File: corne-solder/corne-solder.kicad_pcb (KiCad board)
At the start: 2 copper layers, 133.8 x 91.9 mm, 47 parts, among them J1 Battery Connector, J2 nice!view, SW1 SW_Push, SW10 SW_Push, SW11 SW_Push, SW12 SW_Push, SW13 SW_Push, SW14 SW_Push, SW15 SW_Push, SW16 SW_Push, SW17 SW_Push, SW18 SW_Push, SW19 SW_Push, SW2 SW_Push, SW20 SW_Push, SW21 SW_Push, SW3 SW_Push, SW4 SW_Push, SW5 SW_Push, SW6 SW_Push, SW7 SW_Push, SW8 SW_Push, SW9 SW_Push, U1 ProMicro

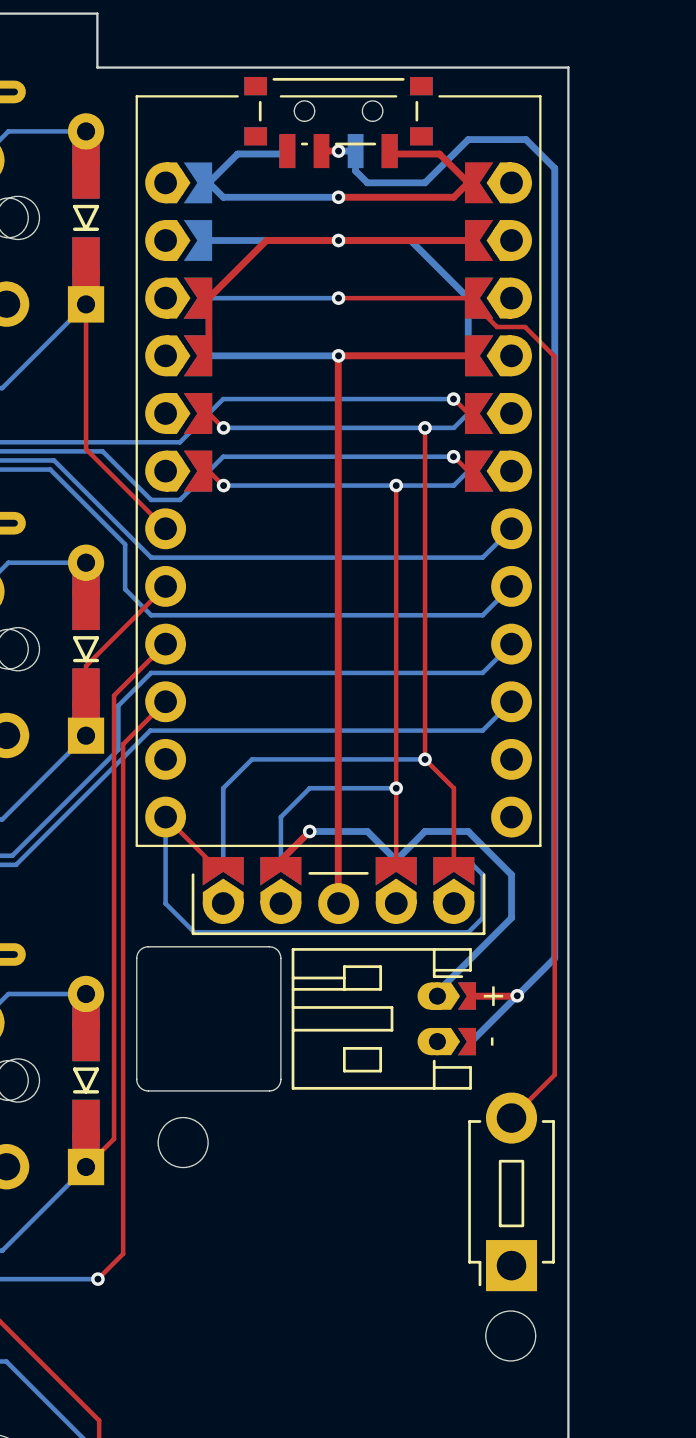
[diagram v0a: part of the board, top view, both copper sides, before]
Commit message: add bridge for wired
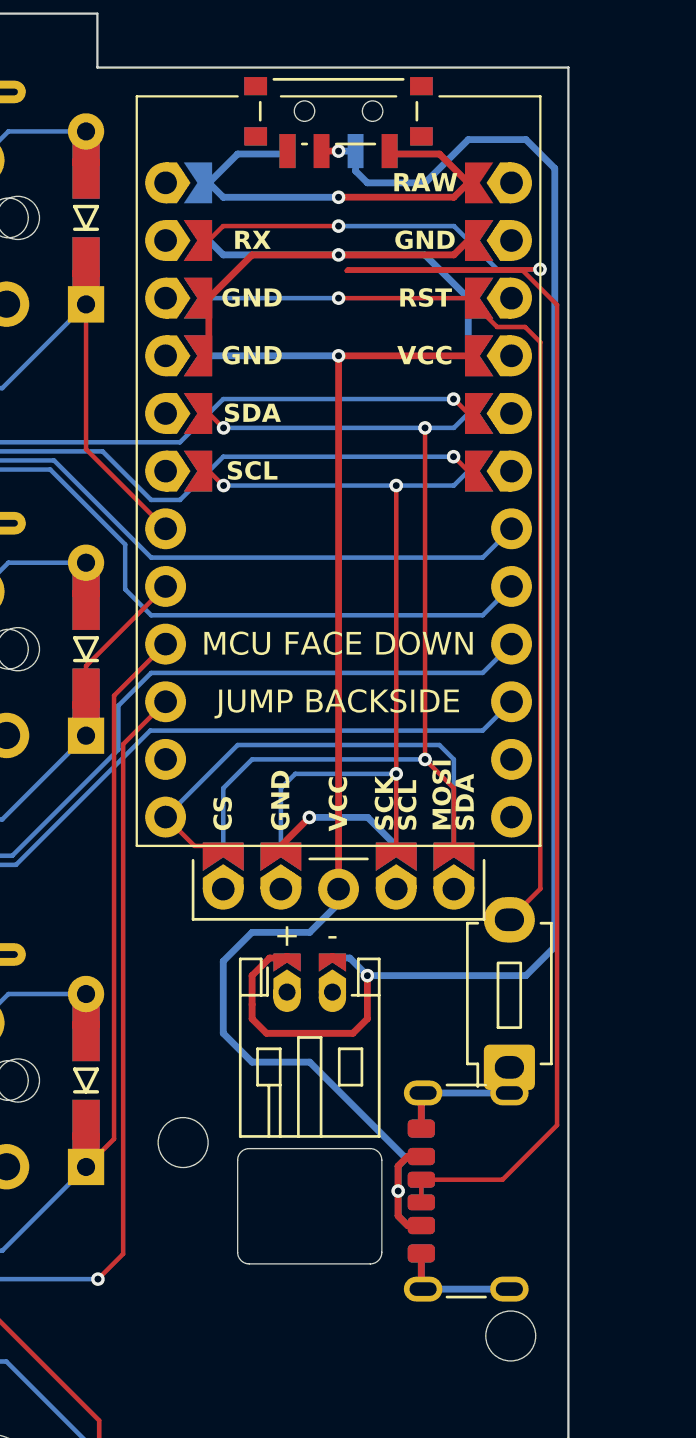
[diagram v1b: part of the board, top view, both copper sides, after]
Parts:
- added J3: USB_C_Receptacle_PowerOnly_6P, Project:USB_C_Receptacle_GCT_USB4125-xx-x_6P_TopMnt_Horizontal, F.Cu at (171.3, 90.5)
- moved RSW1 8.74 mm to (172.2, 85.0)
- moved J1 6.63 mm to (162.4, 81.7), turned to 0 degrees
- moved J2 0.64 mm to (164.6, 77.2)
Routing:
- net RX: track 0.00 -> 79.2 mm, vias 0 -> 2
- net VCC: track 35.6 -> 65.0 mm, vias 1 -> 2
- net Net-(J1-Pin_2): track 54.7 -> 68.9 mm
- net RST: track 50.6 -> 41.4 mm
- net CS: track 25.3 -> 21.2 mm
- net SDA: track 44.1 -> 42.9 mm
- net GND: track 49.3 -> 50.2 mm
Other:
- outline, holes or cut-outs redrawn
